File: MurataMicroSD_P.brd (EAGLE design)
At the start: 25.6 x 12.8 mm, 39 parts, among them U1 IC_BLE_LBCA2HNZYZ-711, U2 IC_BLE_LBCA2HNZYZ-711, U3 IC_BLE_LBCA2HNZYZ-711, U4 IC_BLE_LBCA2HNZYZ-711, U5 IC_BLE_LBCA2HNZYZ-711, U6 IC_BLE_LBCA2HNZYZ-711

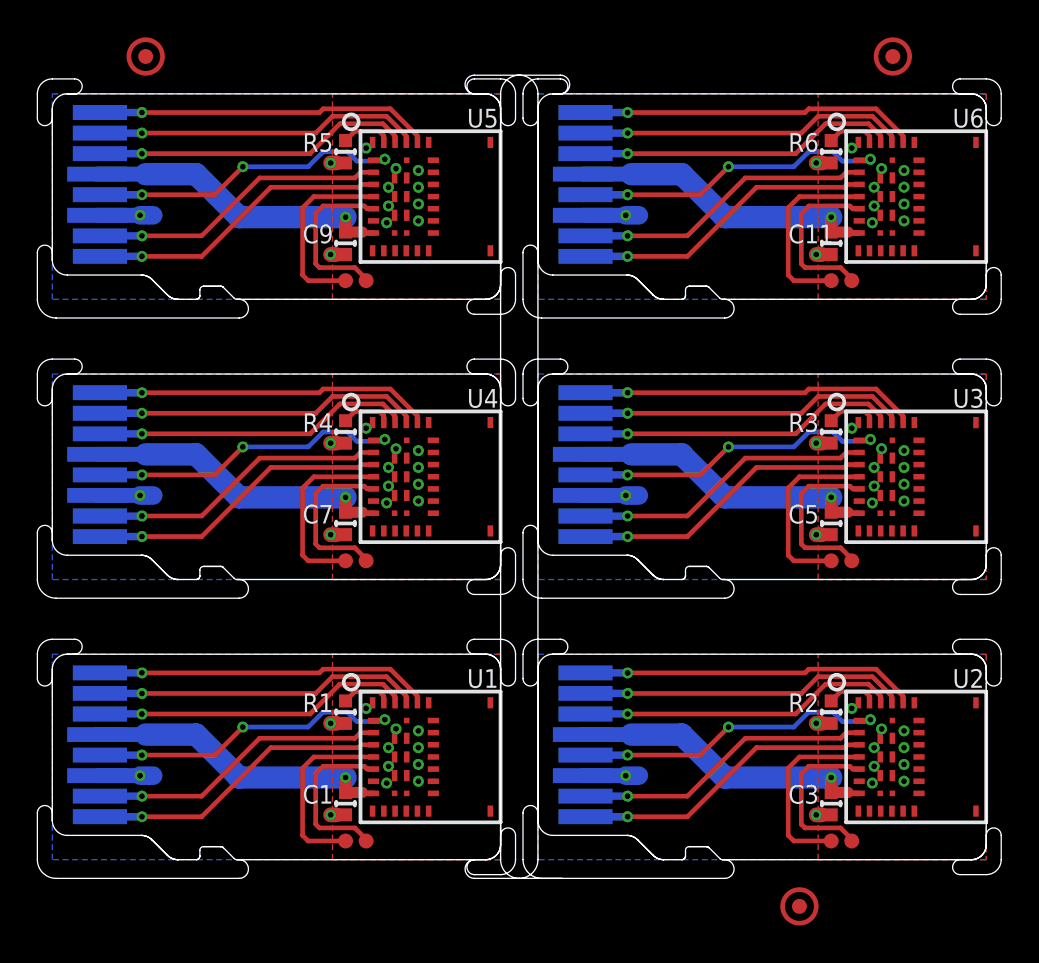
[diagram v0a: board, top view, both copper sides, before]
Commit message: [ uSD ][ GERBER ] panelise as update
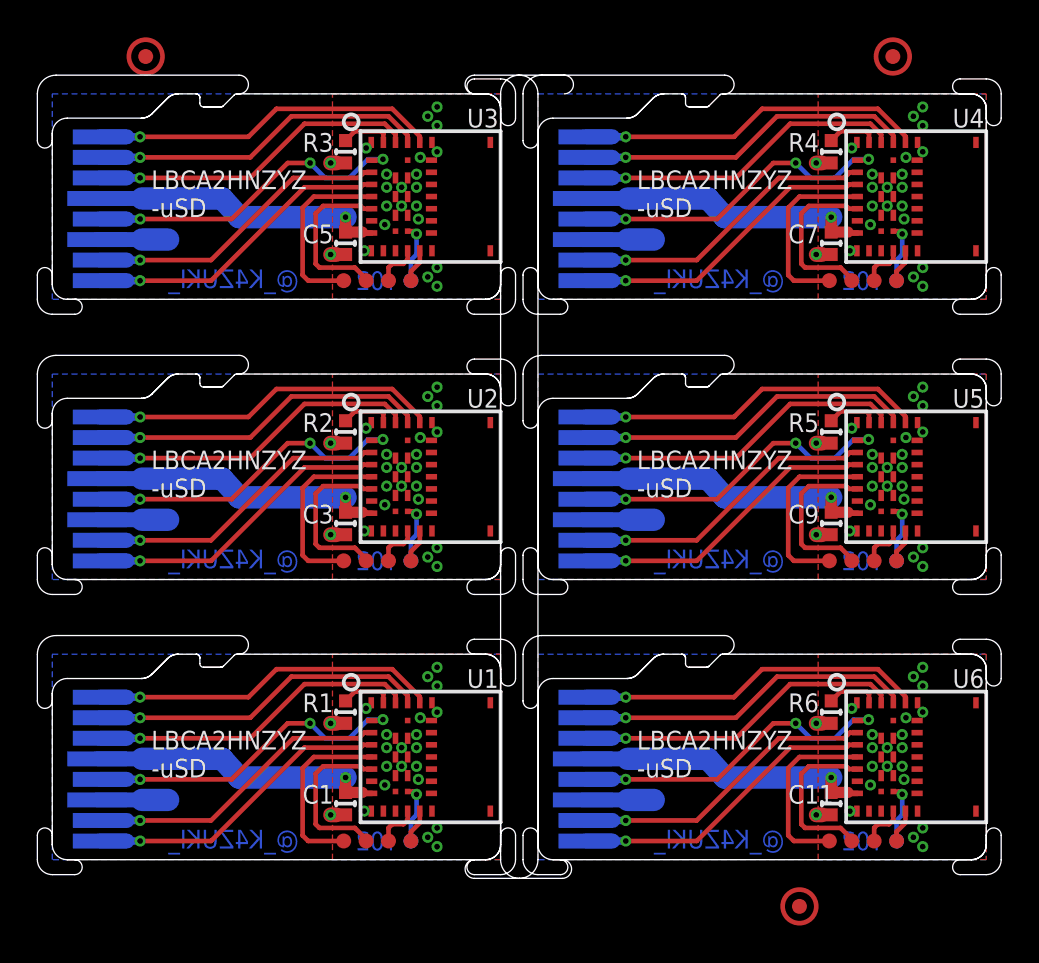
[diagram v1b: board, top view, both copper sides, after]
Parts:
- added TP16, TP17, TP18, TP19, TP20, TP21, TP22, TP23, TP24, TP25, TP26, TP27, TP28, TP29, TP30, TP31, TP32, TP33: TPTP08R, testpad_local:TP08R
- moved C2 36.8 mm to (0.00, 31.0), flipped to the bottom, turned to 180 degrees
- moved C4 36.8 mm to (0.00, 46.0), flipped to the bottom, turned to 180 degrees
- moved C6 36.8 mm to (26.0, 46.0), flipped to the bottom, turned to 180 degrees
- moved C3 30.0 mm to (15.7, 23.0)
- moved C5 30.0 mm to (15.7, 38.0)
- moved C7 30.0 mm to (41.7, 38.0)
- moved C9 30.0 mm to (41.7, 23.0)
- moved R2 30.0 mm to (15.7, 27.9)
- moved R3 30.0 mm to (15.7, 42.9)
- moved R4 30.0 mm to (41.7, 42.9)
- moved R5 30.0 mm to (41.7, 27.9)
- moved U2 30.0 mm to (16.5, 29.0)
- moved U3 30.0 mm to (16.5, 44.0)
- moved U4 30.0 mm to (42.5, 44.0)
- moved U5 30.0 mm to (42.5, 29.0)
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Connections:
- net TXD_MISO renamed MISO
- net TXD_MISO1 renamed MISO1
- net TXD_MISO2 renamed MISO2
- net TXD_MISO3 renamed MISO3
- net TXD_MISO4 renamed MISO4
- net TXD_MISO5 renamed MISO5
- removed net N$3 (its old number): U2.11
- removed net N$5 (its old number): U3.11
- removed net N$7 (its old number): U4.11
- new net N$2: TP6.TP, U1.31
- new net N$4: TP11.TP, U2.31
- new net N$6: TP16.TP, U3.31
- new net P0_1: TP12.TP, U2.11
- new net P0_10: TP28.TP, U5.12
- new net P0_11: TP32.TP, U6.11
- new net P0_12: TP33.TP, U6.12
- new net P0_2: TP8.TP, U1.12
- new net P0_3: TP7.TP, U1.11
- new net P0_4: TP13.TP, U2.12
- new net P0_5: TP17.TP, U3.11
- new net P0_6: TP18.TP, U3.12
- new net P0_7: TP22.TP, U4.11
- new net P0_8: TP23.TP, U4.12
- new net P0_9: TP27.TP, U5.11
- net DAT10: now also C8.1_DAT2, U5.22; no longer C8.8_DAT1, U5.3
- net DAT11: now also C10.8_DAT1, U6.3; no longer C10.1_DAT2, U6.22
- net DAT12: now also C10.1_DAT2, U6.22; no longer C10.8_DAT1, U6.3
- net DAT3: now also C2.8_DAT1, U2.3; no longer C2.1_DAT2, U2.22
- net DAT4: now also C2.1_DAT2, U2.22; no longer C2.8_DAT1, U2.3
- net DAT5: now also C4.8_DAT1, U3.3; no longer C4.1_DAT2, U3.22
- net DAT6: now also C4.1_DAT2, U3.22; no longer C4.8_DAT1, U3.3
- net DAT7: now also C6.8_DAT1, U4.3; no longer C6.1_DAT2, U4.22
- net DAT8: now also C6.1_DAT2, U4.22; no longer C6.8_DAT1, U4.3
- net DAT9: now also C8.8_DAT1, U5.3; no longer C8.1_DAT2, U5.22
- net N$10: now also TP26.TP, U5.31; no longer U5.11
- net N$12: now also TP31.TP, U6.31; no longer U6.11
- net N$8: now also TP21.TP, U4.31; no longer U1.11
- net SWCLK1: now also TP9.TP; no longer TP6.TP
- net SWCLK2: now also TP14.TP; no longer TP8.TP
- net SWCLK3: now also TP19.TP; no longer TP10.TP
- net SWCLK4: now also TP24.TP; no longer TP12.TP
- net SWCLK5: now also TP29.TP; no longer TP14.TP
- net SWDIO1: now also TP10.TP; no longer TP7.TP
- net SWDIO2: now also TP15.TP; no longer TP9.TP
- net SWDIO3: now also TP20.TP; no longer TP11.TP
- net SWDIO4: now also TP25.TP; no longer TP13.TP
- net SWDIO5: now also TP30.TP; no longer TP15.TP
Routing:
- net N$6: track 0.00 -> 3.16 mm, vias 0 -> 1
- net N$4: track 0.00 -> 3.16 mm, vias 0 -> 1
- net N$2: track 0.00 -> 3.16 mm, vias 0 -> 1
- net N$12: track 0.00 -> 3.16 mm, vias 0 -> 1
- net N$8: track 0.00 -> 3.16 mm, vias 0 -> 1
- net N$10: track 0.00 -> 3.16 mm, vias 0 -> 1
- net DAT8: track 16.2 -> 18.7 mm
- net DAT6: track 16.2 -> 18.7 mm
- net DAT4: track 16.2 -> 18.7 mm
- net DAT10: track 16.2 -> 18.7 mm
- net DAT12: track 16.2 -> 18.7 mm
- net P0_5: track 0.00 -> 2.38 mm
- net P0_1: track 0.00 -> 2.38 mm
- net P0_7: track 0.00 -> 2.38 mm
- net P0_3: track 0.00 -> 2.38 mm
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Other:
- outline, holes or cut-outs redrawn
- board text added: "@_K4ZUKI_"
- board text added: "LBCA2HNZYZ -uSD"
- board text added: "r02"
